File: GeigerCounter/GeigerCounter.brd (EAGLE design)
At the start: 100 x 80 mm, 38 parts, among them IC1 OPAMP-DUALU

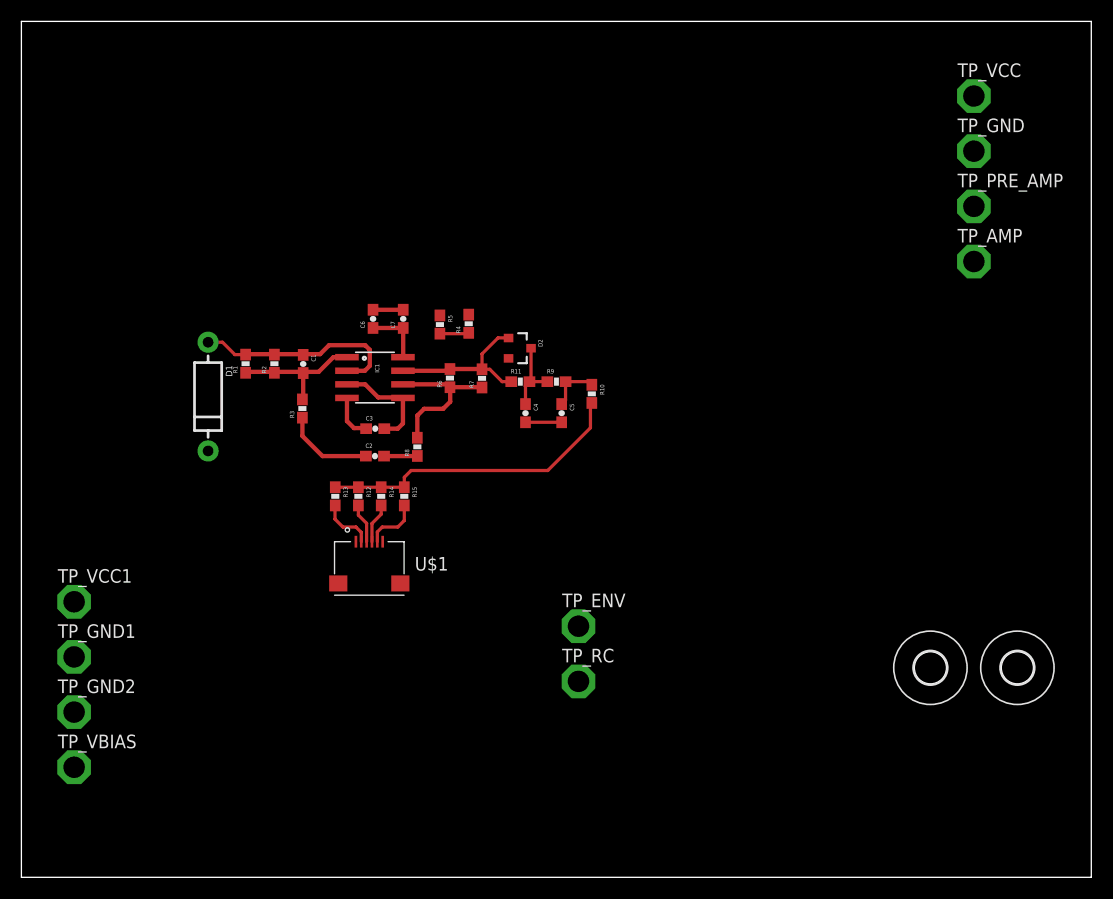
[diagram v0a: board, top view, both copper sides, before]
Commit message: More routing
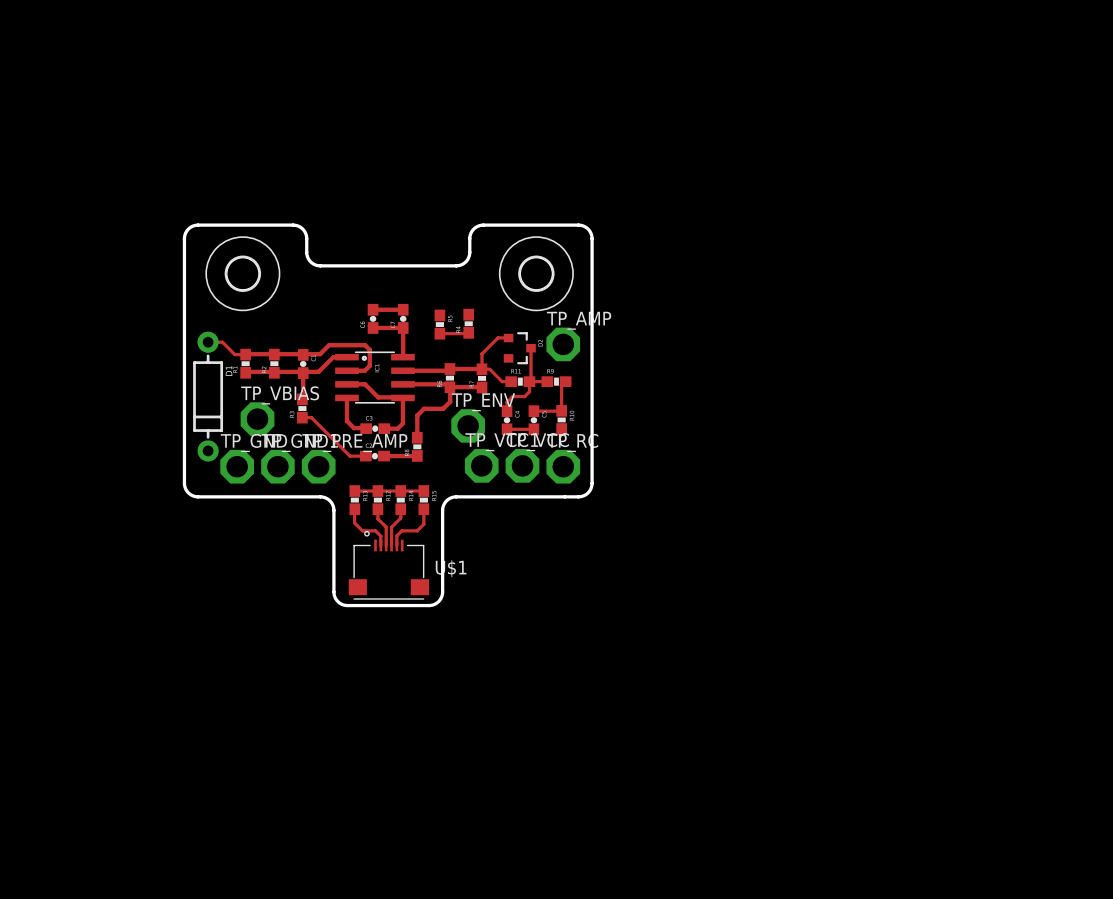
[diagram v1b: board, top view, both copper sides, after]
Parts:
- removed TP_GND2: PTR1PAD1-20, testpad:P1-20
- moved H1 81.2 mm to (20.7, 56.4)
- moved TP_GND 74.9 mm to (20.2, 38.4)
- moved TP_PRE_AMP 65.9 mm to (27.8, 38.4)
- moved TP_VCC 54.5 mm to (46.8, 38.5)
- moved H2 52.1 mm to (48.1, 56.4)
- moved TP_VCC1 40.2 mm to (43.0, 38.5)
- moved TP_AMP 39.2 mm to (50.6, 49.8)
- moved TP_VBIAS 36.8 mm to (22.1, 42.8)
- moved TP_GND1 26.1 mm to (24.0, 38.4)
- moved TP_ENV 21.4 mm to (41.8, 42.2)
- moved TP_RC 20.1 mm to (50.6, 38.4)
- moved R10 3.73 mm to (50.5, 42.7)
- moved C5 2.67 mm to (47.9, 42.7)
- moved R12 1.86 mm to (33.3, 35.3)
- moved U$1 1.86 mm to (34.4, 28.5)
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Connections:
- net GND: no longer TP_GND2.TP
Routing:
- net OUTPUT: track 29.1 -> 6.45 mm
- net ENV_DETEC_OUT: track 7.11 -> 9.15 mm
- net PRE_AMP: track 8.43 -> 7.42 mm
- net GND: track 10.4 -> 9.58 mm
- net RC_OUT: track 4.82 -> 5.48 mm
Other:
- board size 100 x 80 mm -> 38.1 x 35.6 mm
